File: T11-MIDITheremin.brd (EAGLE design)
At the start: 101.6 x 76.2 mm, 102 parts, among them IC1 TL072P, IC2 TL072P, T1 2N3904, T2 2N3904, T3 2N3904, T4 2N3904, T5 2N3904

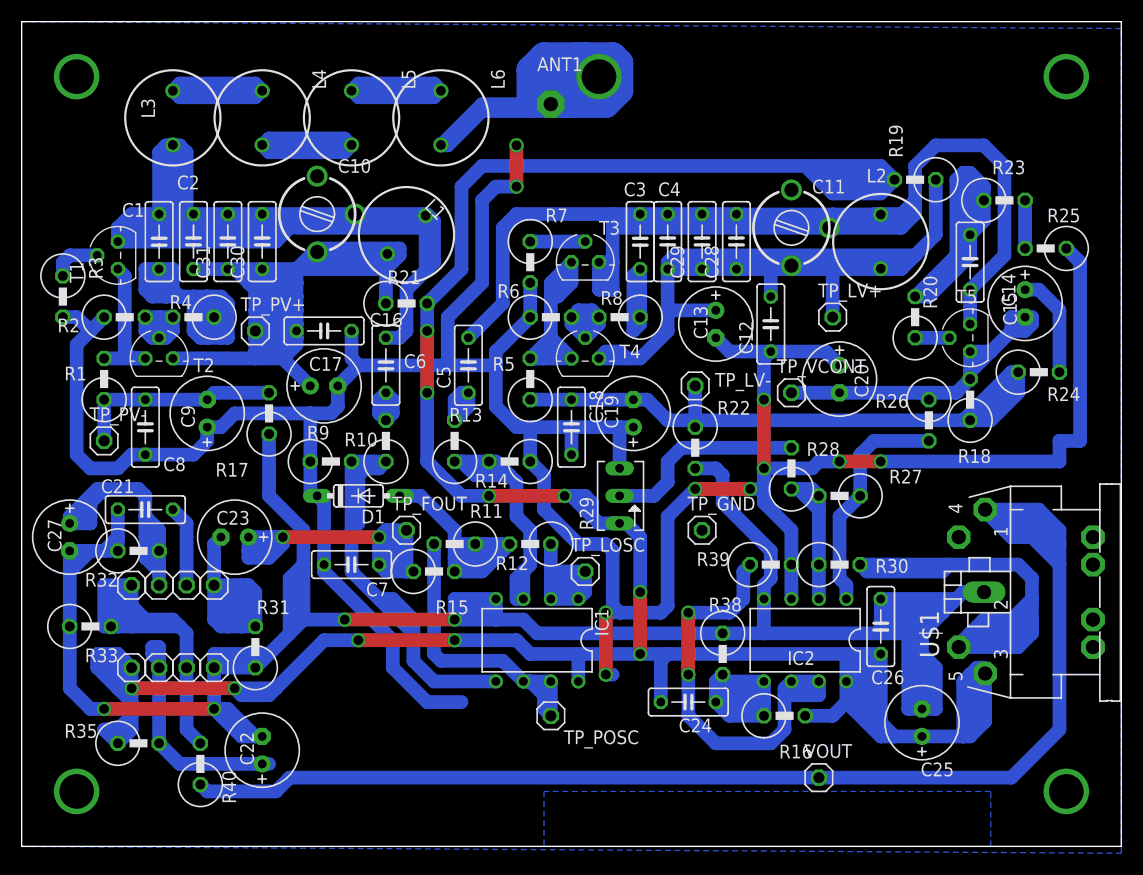
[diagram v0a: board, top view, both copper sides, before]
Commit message: Add files via upload
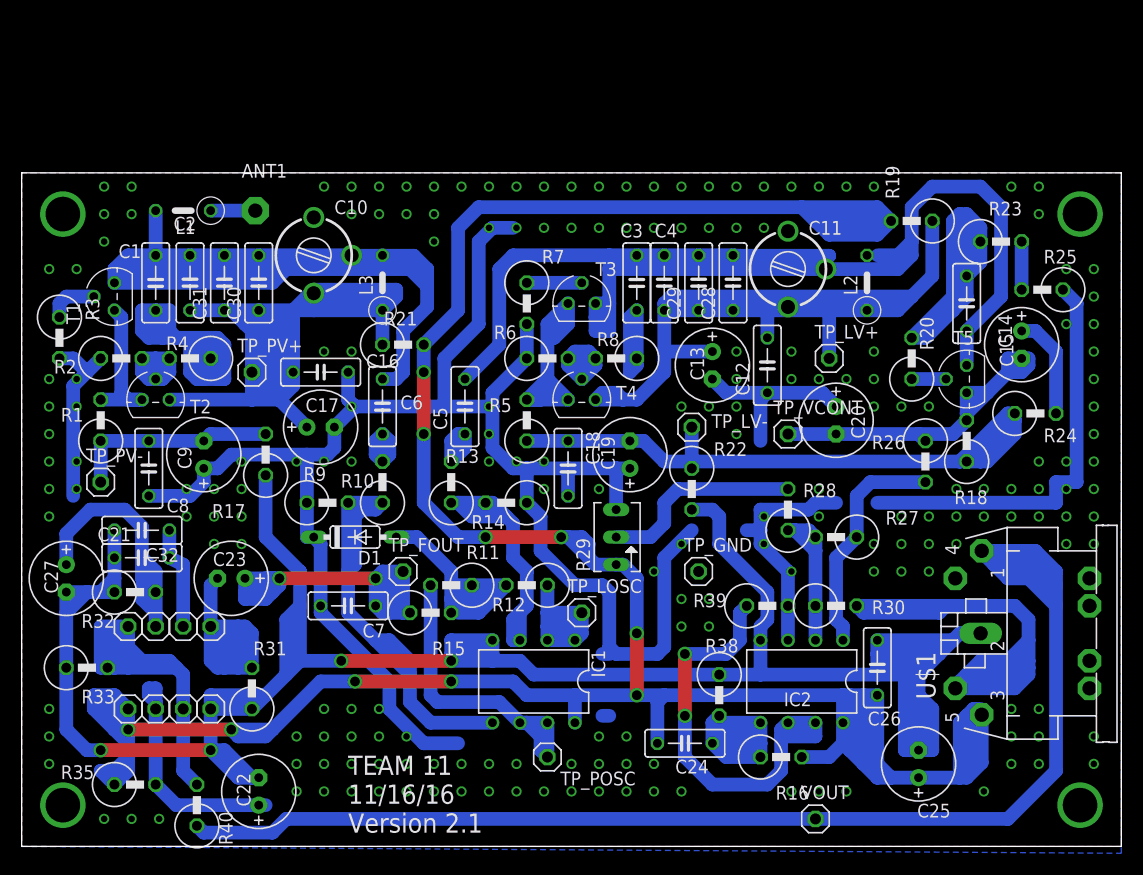
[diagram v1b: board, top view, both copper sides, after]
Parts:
- removed L4, L5, L6: 10mH, rcl:6000-XXXX-RC
- added C32: 2200pF, resistor:C050-025X075
- C2, C4: value 3n3 .1% -> 1.2nF
- L1: value 100uH .1% -> 2.5mH; device rcl:6000-XXXX-RC -> resistor:0207/5V
- L2: value 100uH .1% -> 100uH; device rcl:6000-XXXX-RC -> resistor:0207/5V
- L3: value 10mH -> 100uH; device rcl:6000-XXXX-RC -> resistor:0207/5V
- moved ANT1 29.0 mm to (21.6, 58.7)
- moved L3 24.6 mm to (33.3, 52.1), turned to 90 degrees
- moved L1 20.8 mm to (14.9, 58.7), turned to 180 degrees
- moved C21 4.46 mm to (11.1, 26.7)
- moved L2 4.02 mm to (78.1, 52.1)
- moved C16 3.82 mm to (27.6, 43.8)
- moved C17 3.82 mm to (27.6, 38.7)
- moved C19 3.82 mm to (56.2, 36.2)
- moved C28 3.82 mm to (65.7, 52.1)
- moved C29 3.82 mm to (62.5, 52.1)
- moved C30 3.82 mm to (21.9, 52.1)
- moved C6 3.82 mm to (33.3, 40.6)
- moved LM2917_8 3.82 mm to (17.5, 12.7)
- moved R10 3.82 mm to (33.3, 34.3)
- moved R13 3.82 mm to (39.7, 34.3)
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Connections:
- removed net ANT: ANT1.1, L6.2
- removed net N$19: L5.1, L6.1
- removed net N$35: L4.2, L5.2
- net N$20: now also C32.1
- net N$28: now also ANT1.1, L1.1; no longer L3.1, L4.1
- net P_OSC_V+: now also L3.1; no longer L1.1
- net V-: now also C32.2
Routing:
- net ANT: track 46.4 -> 0.00 mm, vias 1 -> 0
- net GND: track 294.9 -> 262.1 mm, vias 10 -> 196
- net N$42: track 17.6 -> 0.00 mm
- net N$44: track 17.6 -> 0.00 mm
- net N$43: track 17.6 -> 0.00 mm
- net N$38: track 12.1 -> 0.00 mm
- net N$45: track 9.57 -> 0.00 mm
- net N$35: track 8.25 -> 0.00 mm
- net N$19: track 8.25 -> 0.00 mm
- net N$41: track 5.61 -> 0.00 mm
- net LOCAL_RESONANCE: track 125.1 -> 120.0 mm
- net N$28: track 8.26 -> 4.13 mm
- net N$33: track 31.6 -> 27.9 mm
- net N$20: track 7.51 -> 9.67 mm
- net V-: track 233.8 -> 235.7 mm
- added copper zone on layer 1, net GND
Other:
- board size 101.6 x 76.2 mm -> 101.6 x 62.2 mm
- board text added: "TEAM 11 11/16/16 Version 2.1"
- board text removed: "Proximity Sensor V1.0"
